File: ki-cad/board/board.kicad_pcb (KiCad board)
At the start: 2 copper layers, 57.8 x 48.8 mm, 14 parts, among them U1 WEMOS_D1_mini

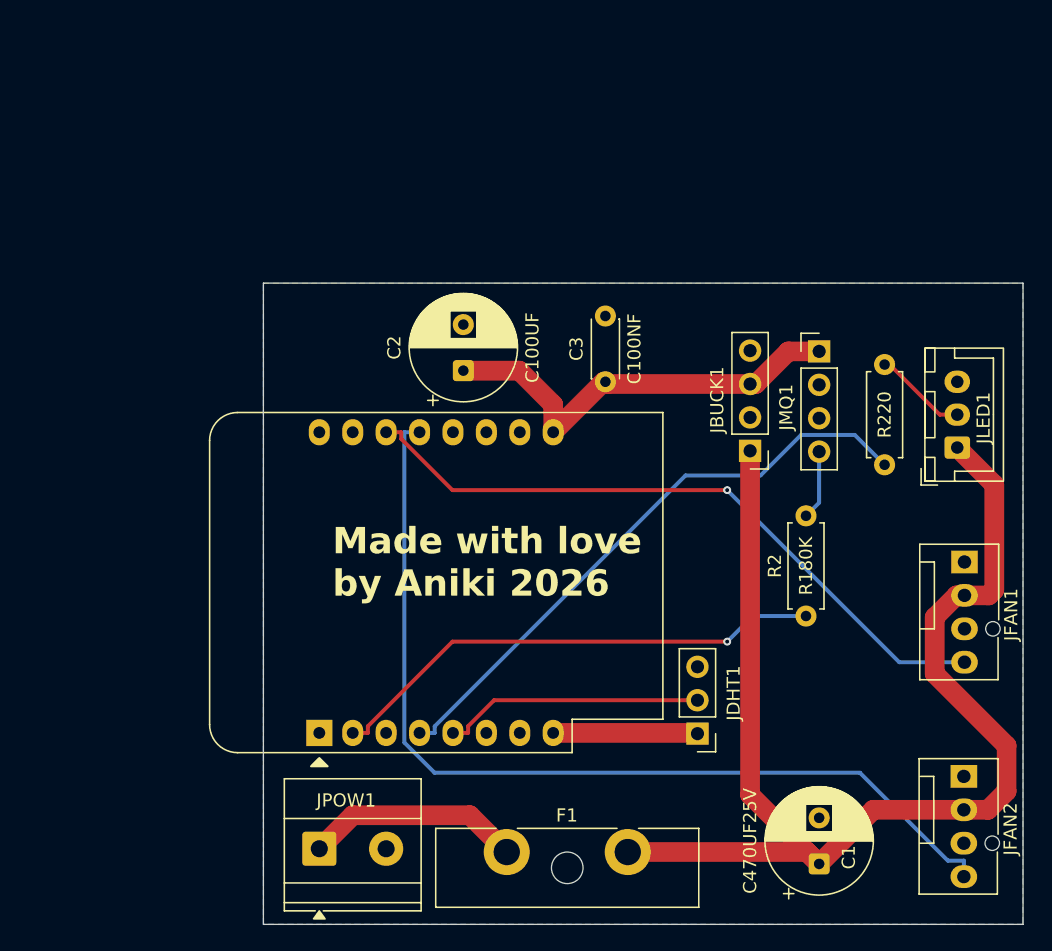
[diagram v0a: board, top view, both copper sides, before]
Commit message: latest ki-cads
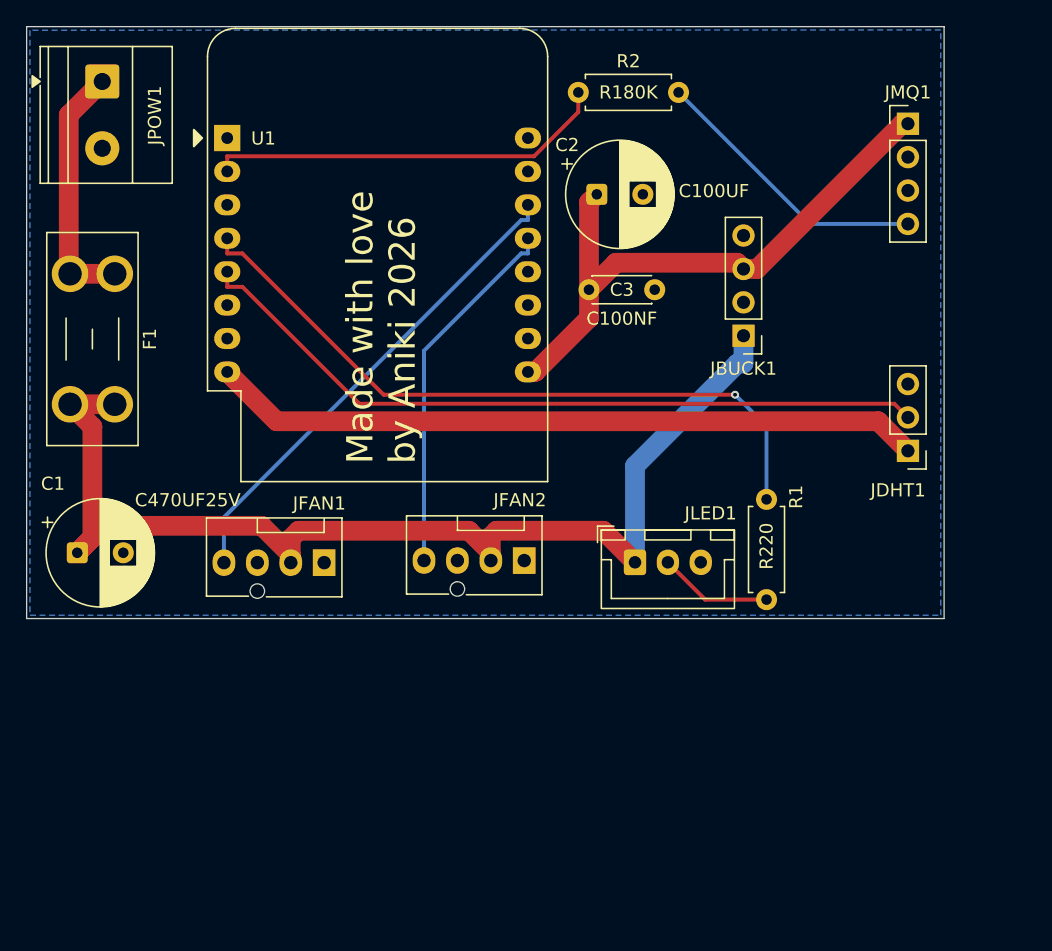
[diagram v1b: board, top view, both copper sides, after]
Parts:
- F1: footprint Fuse:Fuseholder_Blade_ATO_Littelfuse_Pudenz_2_Pin -> Fuse:Fuseholder_Blade_Mini_Keystone_3568
- moved C1 61.2 mm to (98.6, 80.0), turned to 0 degrees
- moved JPOW1 60.6 mm to (100.5, 44.2), turned to -90 degrees
- moved F1 53.1 mm to (101.5, 58.8), turned to -90 degrees
- moved JFAN1 48.7 mm to (117.4, 80.8), turned to 180 degrees
- moved U1 45.8 mm to (110.0, 48.5), turned to 0 degrees
- moved R2 43.4 mm to (136.7, 45.0), turned to 0 degrees
- moved JFAN2 37.2 mm to (132.6, 80.6), turned to 180 degrees
- moved JDHT1 26.8 mm to (161.8, 72.2)
- moved JLED1 26.0 mm to (141.0, 80.7), turned to 0 degrees
- moved R1 20.0 mm to (151.0, 83.6), turned to 90 degrees
- moved JMQ1 18.6 mm to (161.8, 47.4)
- moved C2 16.8 mm to (138.1, 52.8), turned to 0 degrees
- moved JBUCK1 8.76 mm to (149.2, 63.5)
- moved C3 7.11 mm to (137.5, 60.0), turned to 0 degrees
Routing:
- net /PWM_2: track 72.2 -> 28.1 mm
- net +3.3V: track 11.0 -> 54.2 mm
- net /DHT_DATA: track 19.9 -> 57.0 mm
- net /AO: track 5.29 -> 21.6 mm
- net /PWM_1: track 51.5 -> 37.1 mm, vias 1 -> 0
- net +5V: track 32.9 -> 45.9 mm
- net +12V: track 97.9 -> 87.9 mm
- net /AO_R: track 38.4 -> 30.7 mm, vias 1 -> 0
- net /LED_DATA: track 46.0 -> 53.2 mm, vias 0 -> 1
- net Net-(JPOW1-Pin_1): track 16.5 -> 19.1 mm
- net /LED_R: track 7.10 -> 8.67 mm
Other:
- board size 57.8 x 48.8 mm -> 69.8 x 45 mm
